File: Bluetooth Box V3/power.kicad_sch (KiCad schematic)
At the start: 8 parts, among them U6 MIC5356-SGYMME

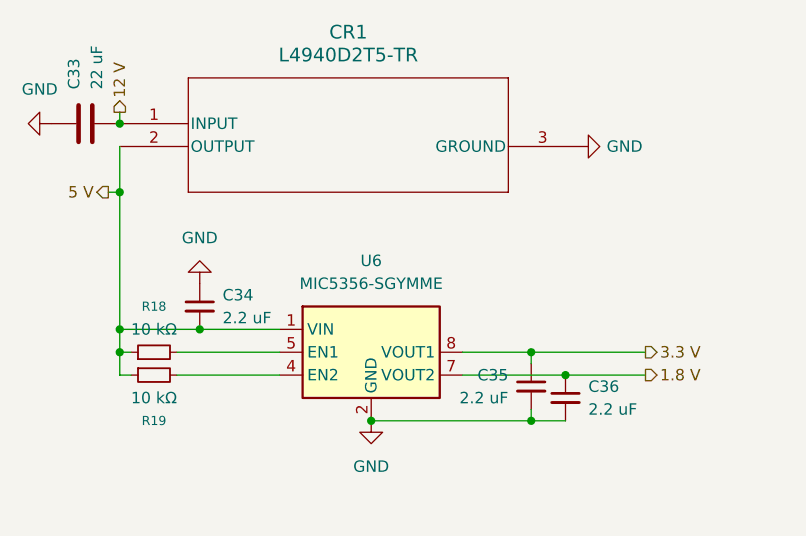
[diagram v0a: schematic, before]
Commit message: Idiotencheck 1
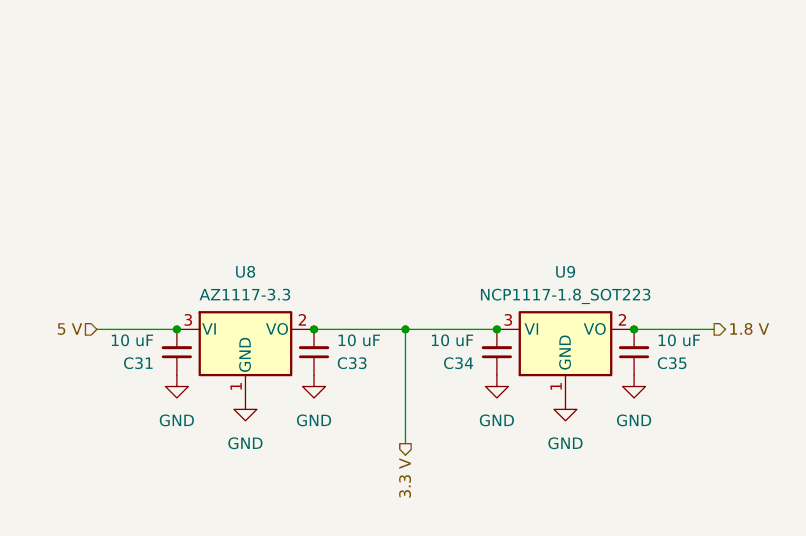
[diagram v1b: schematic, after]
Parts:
- removed C33: 22 uF, Capacitor_SMD:C_0805_2012Metric, symbol Device:C
- removed C36: 2.2 uF, Capacitor_SMD:C_0805_2012Metric, symbol Device:C_Small
- removed CR1: L4940D2T5-TR, ul_L4940D2T5-TR:D2PAK_STM, symbol 2026-02-19_20-19-44:L4940D2T5-TR
- removed R18, R19: 10 kΩ, Resistor_SMD:R_0805_2012Metric, symbol Device:R_Small
- removed U6: MIC5356-SGYMME, Package_SO:MSOP-8-1EP_3x3mm_P0.65mm_EP2.5x3mm_Mask1.73x2.36mm_ThermalVias, symbol Regulator_Linear:MIC5356-SGYMME
- added C31, C33: 10 uF, Capacitor_SMD:C_0805_2012Metric, symbol Device:C_Small
- added U8: AZ1117-3.3, Package_TO_SOT_SMD:TO-252-2, symbol Regulator_Linear:AZ1117-3.3
- added U9: NCP1117-1.8_SOT223, Package_TO_SOT_SMD:SOT-223-3_TabPin2, symbol Regulator_Linear:NCP1117-1.8_SOT223
- C34, C35: value 2.2 uF -> 10 uF; LCSC Part # C377773 -> C440198
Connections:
- net 1.8 V: now also C35.2, U9.2 (VO)
- net 3.3 V: now also C34.2, C33.2, U8.2 (VO), U9.3 (VI); no longer C35.1
- net 5 V: now also C31.2, U8.3 (VI); no longer C34.2
- net GND: now also C35.1, C31.1, C33.1, U8.1 (GND), U9.1 (GND); no longer C35.2
